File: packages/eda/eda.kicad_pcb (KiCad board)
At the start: 2 copper layers, 38 parts, among them U1 Pico

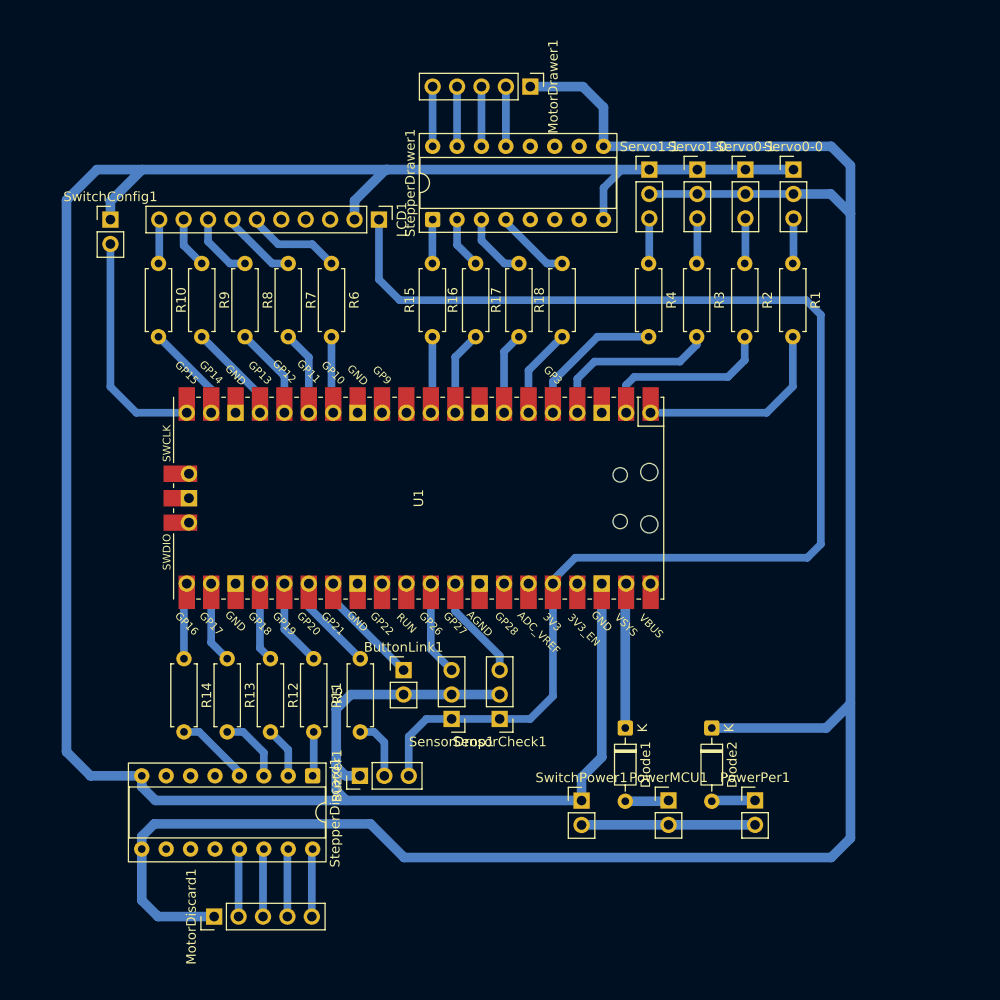
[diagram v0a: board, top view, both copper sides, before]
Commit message: chore: bump deps
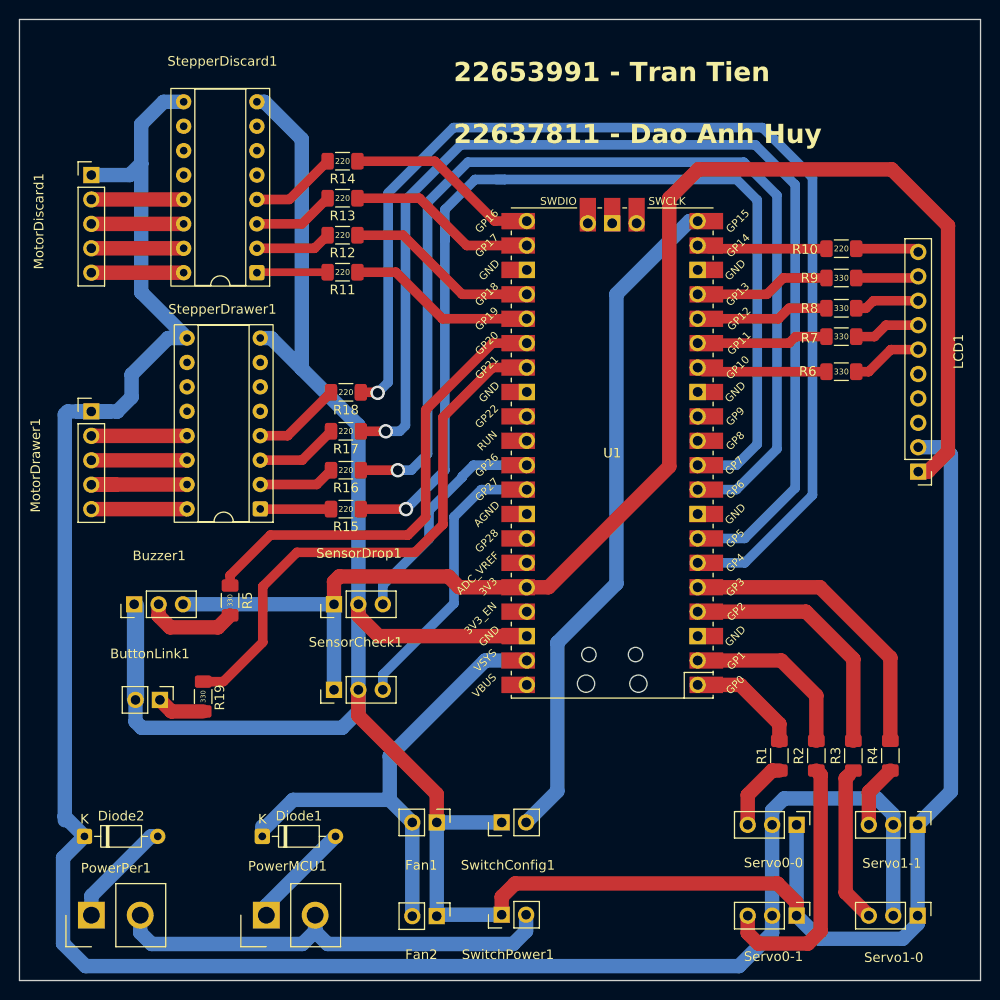
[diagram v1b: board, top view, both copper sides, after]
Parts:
- added Fan1: ~, Connector_PinHeader_2.54mm:PinHeader_1x02_P2.54mm_Vertical, F.Cu at (152.9, 134.3)
- added Fan2: ~, Connector_PinHeader_2.54mm:PinHeader_1x02_P2.54mm_Vertical, F.Cu at (152.9, 144.1)
- added R19: 330, Resistor_SMD:R_1206_3216Metric_Pad1.30x1.75mm_HandSolder, F.Cu at (128.7, 121.2)
- PowerMCU1, PowerPer1: footprint Connector_PinHeader_2.54mm:PinHeader_1x02_P2.54mm_Vertical -> Connector_Samtec_HPM_THT:Samtec_HPM-02-01-x-S_Straight_1x02_Pitch5.08mm
- R1, R10, R11, R12, R13, R14, R15, R16, R17, R18, R2, R3, R4, R5, R6, R7, R8, R9: footprint Resistor_THT:R_Axial_DIN0207_L6.3mm_D2.5mm_P7.62mm_Horizontal -> Resistor_SMD:R_1206_3216Metric_Pad1.30x1.75mm_HandSolder
- moved Servo1-0 80.9 mm to (203.0, 144.1), turned to -90 degrees
- moved MotorDiscard1 78.2 mm to (117.0, 67.0), turned to 0 degrees
- moved Servo0-1 77.8 mm to (190.4, 144.1), turned to -90 degrees
- moved SwitchConfig1 74.8 mm to (159.7, 134.3), turned to 90 degrees
- moved Servo1-1 73.7 mm to (203.0, 134.6), turned to -90 degrees
- moved R10 71.1 mm to (195.1, 74.7), turned to 180 degrees
- moved PowerPer1 70.1 mm to (117.0, 144.0), turned to 90 degrees
- moved Servo0-0 68.2 mm to (190.4, 134.6), turned to -90 degrees
- moved R9 66.6 mm to (195.1, 77.7), turned to 180 degrees
- moved Diode2 66.2 mm to (116.3, 135.8), turned to 0 degrees
- moved R8 62.2 mm to (195.1, 80.8), turned to 180 degrees
- moved LCD1 61.9 mm to (203.1, 97.8), turned to 180 degrees
- moved R7 58.1 mm to (195.1, 83.8), turned to 180 degrees
- moved R4 57.1 mm to (200.2, 127.4), turned to 90 degrees
- moved MotorDrawer1 56.8 mm to (117.0, 91.6), turned to 0 degrees
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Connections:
- ButtonLink1 pad 1: /BTN -> Net-(ButtonLink1-Pin_1)
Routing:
- net /StD11: track 9.36 -> 120.1 mm, vias 0 -> 1
- net /StD12: track 8.55 -> 116.9 mm, vias 0 -> 1
- net /StD13: track 9.17 -> 109.7 mm, vias 0 -> 1
- net /StD14: track 8.36 -> 106.6 mm, vias 0 -> 1
- net /SW: track 23.9 -> 70.5 mm
- net /BTN: track 12.0 -> 57.1 mm
- net /Buzzer: track 10.0 -> 48.5 mm
- net /VCC: track 15.1 -> 51.6 mm
- net /GNDP: track 18.2 -> 49.2 mm
- net Net-(Servo0-1-Pin_3): track 4.62 -> 27.3 mm
- net /SC: track 10.9 -> 29.8 mm
- net /Serv11: track 15.1 -> 31.2 mm
- net /3.3V: track 139.9 -> 155.8 mm
- net /SD: track 9.89 -> 23.9 mm
- net /GND: track 269.5 -> 283.4 mm
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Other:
- board outline added: 100 x 100 mm
- board text added: "22653991 - Tran Tien 22637811 - Dao Anh Huy"
